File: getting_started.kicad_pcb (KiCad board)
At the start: 2 copper layers, 17 x 26 mm, 12 parts, among them J1 Conn_01x04_Pin, J2 Conn_ARM_JTAG_SWD_10, U1 STM32F030F4Px, U2 SHT4x

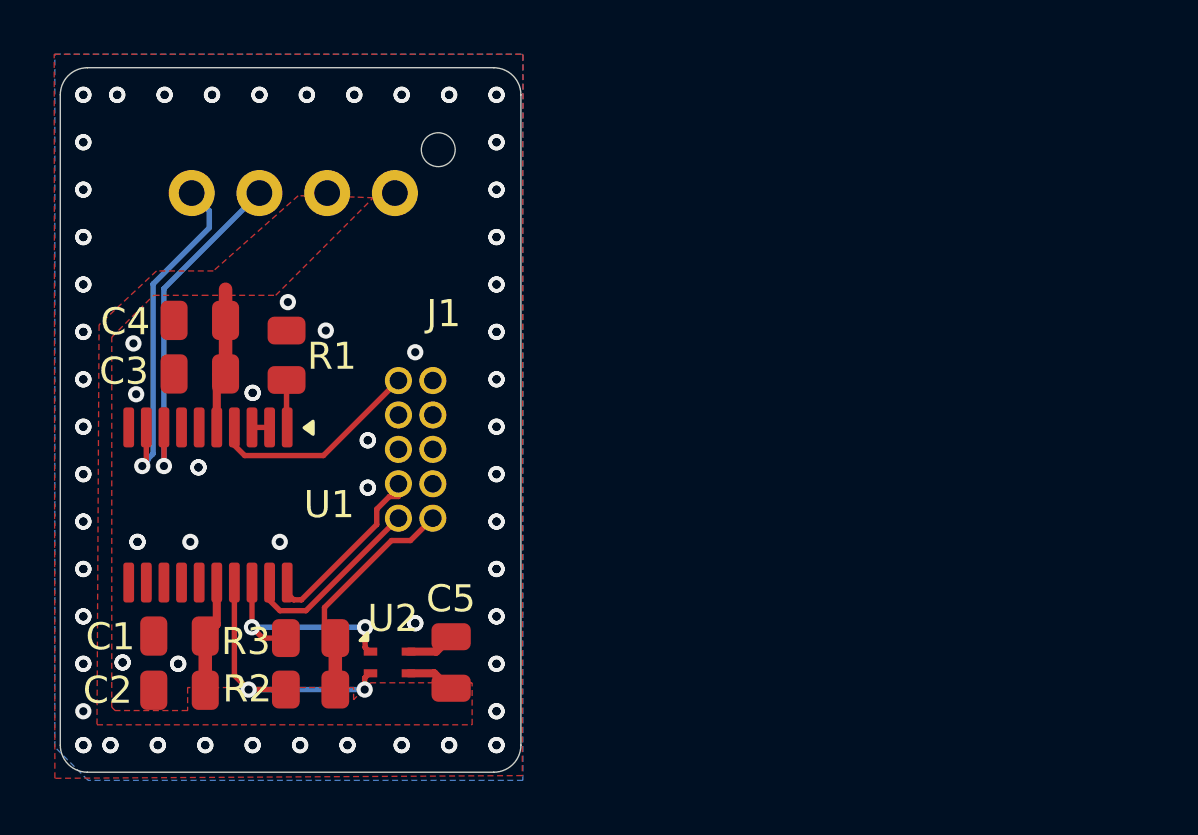
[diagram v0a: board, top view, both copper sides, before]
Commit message: Pass ERC and DRC
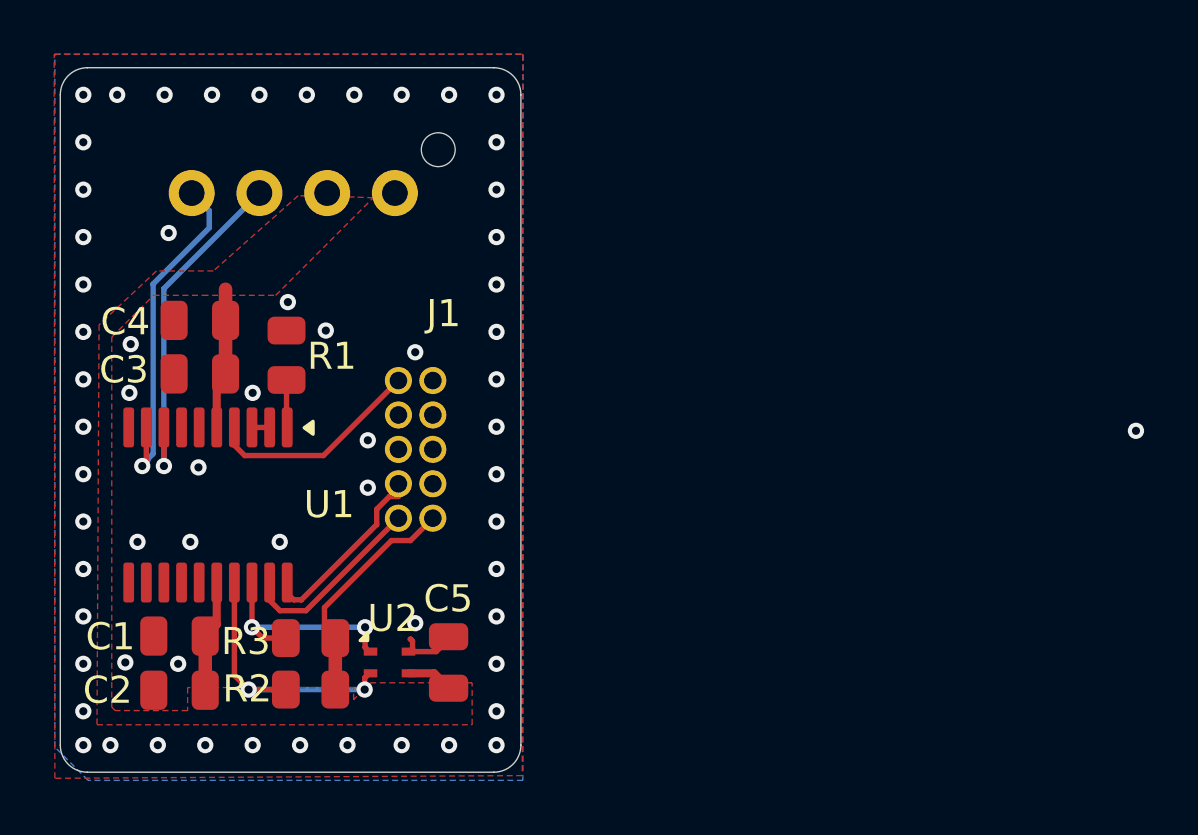
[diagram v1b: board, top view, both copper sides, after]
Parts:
- moved C5 0.09 mm to (117.7, 122.5)
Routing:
- net GND: track 2.52 -> 3.12 mm, vias 114 -> 62
- net (no net): vias 0 -> 1
